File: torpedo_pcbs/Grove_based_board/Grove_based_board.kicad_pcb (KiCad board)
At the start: 2 copper layers, 85 x 27.5 mm, 11 parts, among them IC1 ICM-20948, J1 503480-2200, J2 503480-2200, J3 503480-0440, J4 503480-0440, J5 S8B-EH

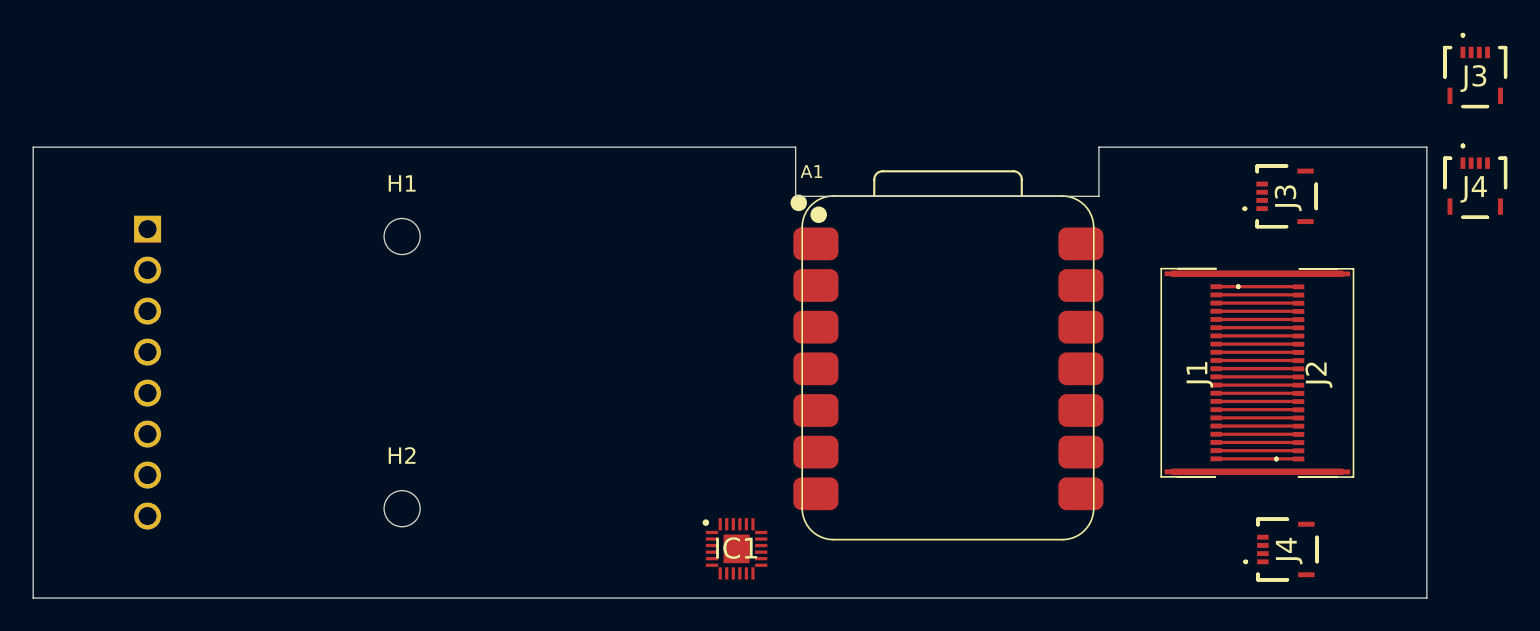
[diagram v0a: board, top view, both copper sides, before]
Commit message: save feb21
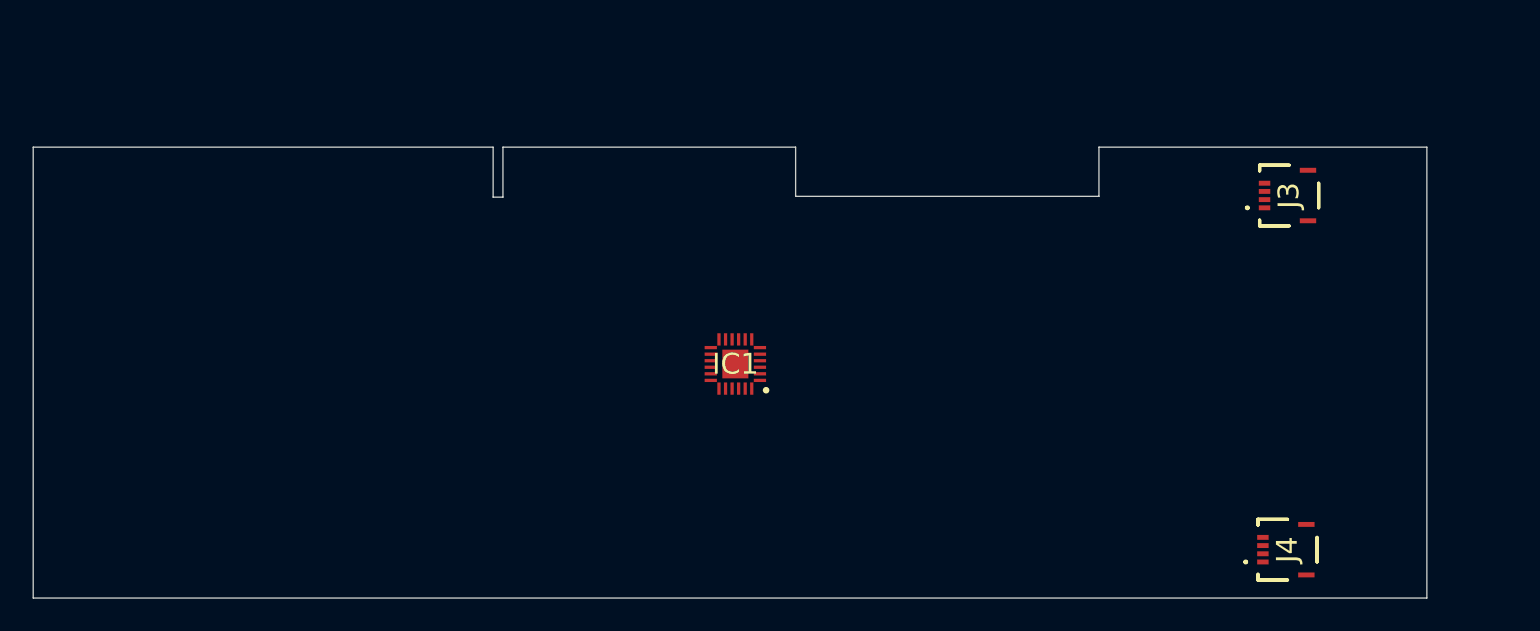
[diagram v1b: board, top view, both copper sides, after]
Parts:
- removed A1: XIAO ESP32S3, board_board_connection:XIAO ESP32S3 SMD
- removed H1, H2: MountingHole, MountingHole:MountingHole_2.2mm_M2
- removed J1, J2: 503480-2200, SamacSys_Parts:5034802200
- removed the J3 at (176.4, 85.0)
- removed the J3 at (187.9, 77.7)
- removed the J4 at (187.9, 84.5)
- removed the J4 at (176.5, 106.5)
- removed J5: S8B-EH, SamacSys_Parts:SHDRRA8W64P0X250_1X8_2250X820X420P
- added J3: 503480-0440, SamacSys_Parts:5034800440, F.Cu at (176.6, 85.0)
- added J4: 503480-0440, SamacSys_Parts:5034800440, F.Cu at (176.5, 106.5)
- moved IC1 11.3 mm to (142.8, 95.2), turned to 180 degrees
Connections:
- IC1 pad 10: unconnected-(IC1-REGOUT-Pad10) -> Net-(IC1-REGOUT)
- IC1 pad 11: unconnected-(IC1-FSYNC-Pad11) -> GND
- IC1 pad 12: unconnected-(IC1-INT1-Pad12) -> IMU_INT
- IC1 pad 13: unconnected-(IC1-VDD-Pad13) -> +3.3V
- IC1 pad 18: unconnected-(IC1-GND-Pad18) -> GND
- IC1 pad 20: unconnected-(IC1-RESV_2-Pad20) -> GND
- IC1 pad 22: unconnected-(IC1-NCS-Pad22) -> +3.3V
- IC1 pad 23: unconnected-(IC1-SCL_/_SCLK-Pad23) -> SCL2
- IC1 pad 24: unconnected-(IC1-SDA_/_SDI-Pad24) -> SDA2
- IC1 pad 8: unconnected-(IC1-VDDIO-Pad8) -> +1V8
- IC1 pad 9: unconnected-(IC1-SDO_/_AD0-Pad9) -> GND
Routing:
- net GND: track 20.7 -> 0.00 mm
- net Net-(J1-Pad1): track 5.03 -> 0.00 mm
- net Net-(J1-Pad9): track 5.02 -> 0.00 mm
- net Net-(J1-Pad8): track 5.02 -> 0.00 mm
- net Net-(J1-Pad7): track 5.02 -> 0.00 mm
- net Net-(J1-Pad6): track 5.02 -> 0.00 mm
- net Net-(J1-Pad5): track 5.02 -> 0.00 mm
- net Net-(J1-Pad4): track 5.02 -> 0.00 mm
- net Net-(J1-Pad3): track 5.02 -> 0.00 mm
- net Net-(J1-Pad22): track 5.02 -> 0.00 mm
- net Net-(J1-Pad21): track 5.02 -> 0.00 mm
- net Net-(J1-Pad20): track 5.02 -> 0.00 mm
- net Net-(J1-Pad2): track 5.02 -> 0.00 mm
- net Net-(J1-Pad19): track 5.02 -> 0.00 mm
- net Net-(J1-Pad18): track 5.02 -> 0.00 mm
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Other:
- outline, holes or cut-outs redrawn
- copper layers 2 -> 4

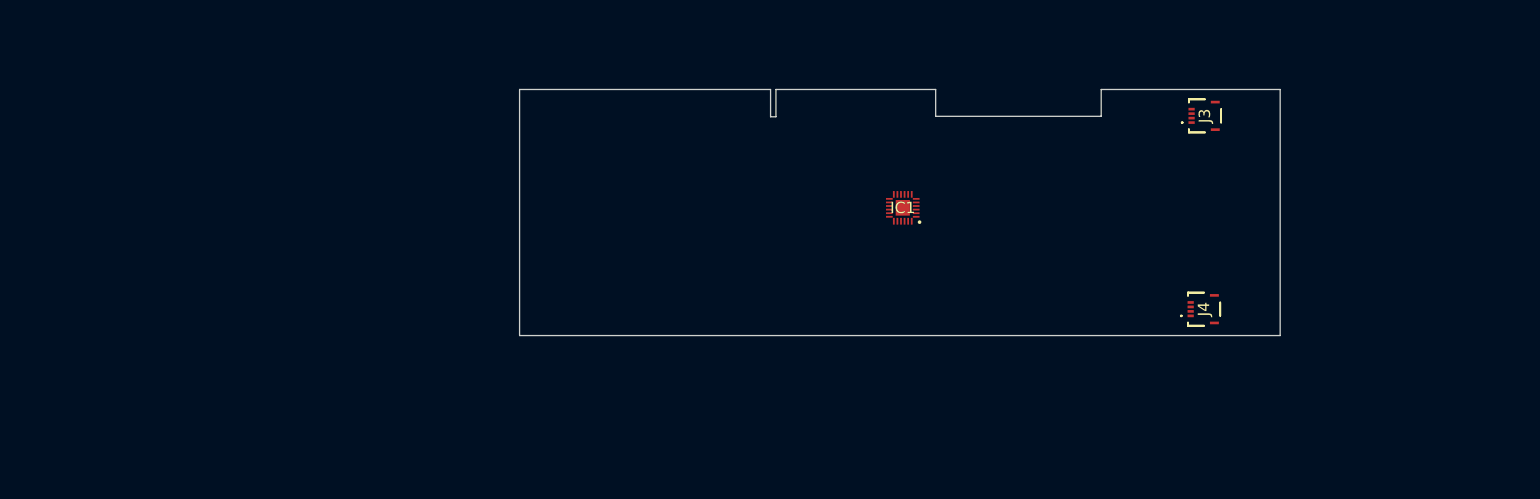
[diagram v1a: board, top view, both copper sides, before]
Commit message: feb23 updates
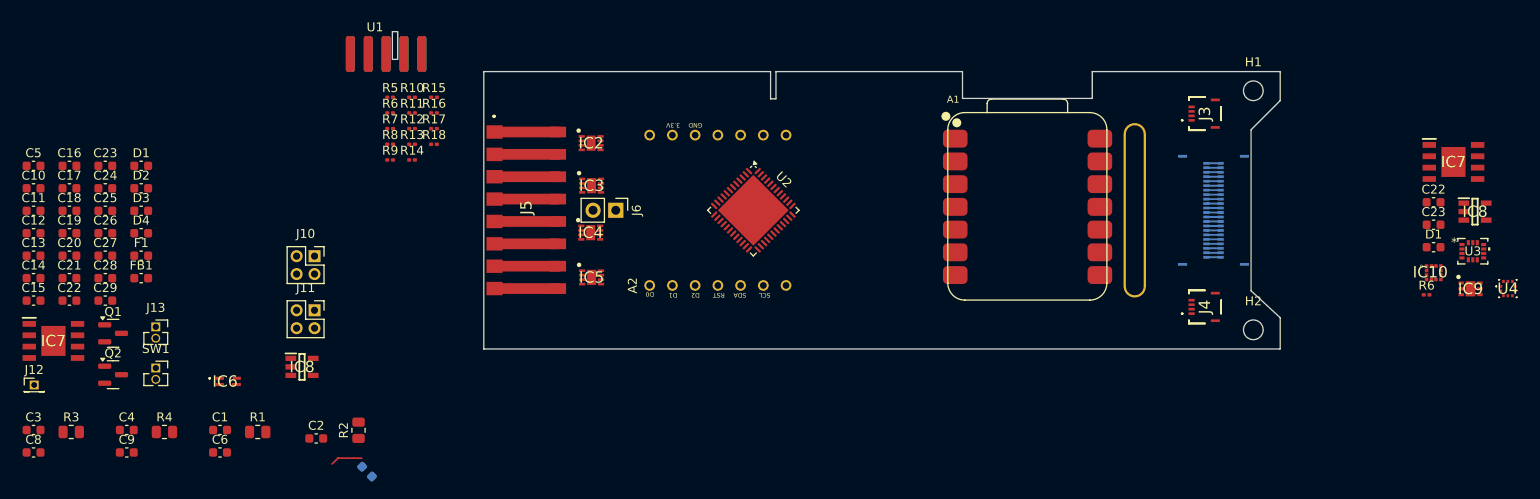
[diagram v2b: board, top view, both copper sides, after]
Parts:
- removed IC1: ICM-20948, SamacSys_Parts:QFN40P300X300X105-25N-D
- added A1: XIAO ESP32S3, board_board_connection:XIAO ESP32S3 SMD, F.Cu at (156.8, 95.1)
- added A2: Grove AI Vision Module V2, board_board_connection:Grove conn, F.Cu at (114.5, 95.5)
- added C1: 0.1μF, Capacitor_SMD:C_0603_1608Metric, F.Cu at (66.5, 120.1)
- added C10: 1μF, Capacitor_SMD:C_0603_1608Metric, F.Cu at (45.7, 93.0)
- added C11: 2.2μF, Capacitor_SMD:C_0603_1608Metric, F.Cu at (45.7, 95.6)
- added C12: 0.1μF, Capacitor_SMD:C_0603_1608Metric, F.Cu at (45.7, 98.1)
- added C13: 10μF, Capacitor_SMD:C_0603_1608Metric, F.Cu at (45.7, 100.6)
- added C14: 0.1μF, Capacitor_SMD:C_0603_1608Metric, F.Cu at (45.7, 103.1)
- added C15: 0.1μF, Capacitor_SMD:C_0603_1608Metric, F.Cu at (45.7, 105.6)
- added C16: 0.1μF, Capacitor_SMD:C_0603_1608Metric, F.Cu at (49.7, 90.5)
- added C17: 0.1μF, Capacitor_SMD:C_0603_1608Metric, F.Cu at (49.7, 93.0)
- added C18: 1μF, Capacitor_SMD:C_0603_1608Metric, F.Cu at (49.7, 95.6)
- added C19: 10nF, Capacitor_SMD:C_0603_1608Metric, F.Cu at (49.7, 98.1)
- added C2: 0.1μF, Capacitor_SMD:C_0603_1608Metric, F.Cu at (77.3, 121.0)
- added C20: 1μF, Capacitor_SMD:C_0603_1608Metric, F.Cu at (49.7, 100.6)
- added C21: 0.1μF, Capacitor_SMD:C_0603_1608Metric, F.Cu at (49.7, 103.1)
- added C22: 10μF, Capacitor_SMD:C_0603_1608Metric, F.Cu at (202.1, 94.6)
- added C22: 10μF, Capacitor_SMD:C_0603_1608Metric, F.Cu at (49.7, 105.6)
- added C23: 10μF, Capacitor_SMD:C_0603_1608Metric, F.Cu at (202.1, 97.1)
- added C23: 10μF, Capacitor_SMD:C_0603_1608Metric, F.Cu at (53.7, 90.5)
- added C24: ??μF, Capacitor_SMD:C_0603_1608Metric, F.Cu at (53.7, 93.0)
- added C25: 1μF, Capacitor_SMD:C_0603_1608Metric, F.Cu at (53.7, 95.6)
- added C26: ??μF, Capacitor_SMD:C_0603_1608Metric, F.Cu at (53.7, 98.1)
- added C27: 0.1μF, Capacitor_SMD:C_0603_1608Metric, F.Cu at (53.7, 100.6)
- added C28: 22nF, Capacitor_SMD:C_0603_1608Metric, F.Cu at (53.7, 103.1)
- added C29: 22nF, Capacitor_SMD:C_0603_1608Metric, F.Cu at (53.7, 105.6)
- added C3: 0.1μF, Capacitor_SMD:C_0603_1608Metric, F.Cu at (45.7, 120.1)
- added C4: 0.1μF, Capacitor_SMD:C_0603_1608Metric, F.Cu at (56.1, 120.1)
- added C5: 0.1μF, Capacitor_SMD:C_0603_1608Metric, F.Cu at (45.7, 90.5)
- added C6: 47μF, Capacitor_SMD:C_0603_1608Metric, F.Cu at (66.5, 122.6)
- added C7: 47μF, Capacitor_SMD:C_0603_1608Metric, B.Cu at (83.0, 124.7)
- added C8: 47μF, Capacitor_SMD:C_0603_1608Metric, F.Cu at (45.7, 122.6)
- added C9: 47μF, Capacitor_SMD:C_0603_1608Metric, F.Cu at (56.1, 122.6)
- added D1: LED, Capacitor_SMD:C_0603_1608Metric, F.Cu at (57.7, 90.5)
- added D1: LED, Capacitor_SMD:C_0603_1608Metric, F.Cu at (202.1, 99.6)
- added D2: LED, Capacitor_SMD:C_0603_1608Metric, F.Cu at (57.7, 93.0)
- added D3: LED, Capacitor_SMD:C_0603_1608Metric, F.Cu at (57.7, 95.6)
- added D4: LED, Capacitor_SMD:C_0603_1608Metric, F.Cu at (57.7, 98.1)
- added F1: Fuse, Capacitor_SMD:C_0603_1608Metric, F.Cu at (57.7, 100.6)
- added FB1: FerriteBead, Capacitor_SMD:C_0603_1608Metric, F.Cu at (57.7, 103.1)
- added H1: MountingHole, MountingHole:MountingHole_2.2mm_M2, F.Cu at (182.0, 82.1)
- added H2: MountingHole, MountingHole:MountingHole_2.2mm_M2, F.Cu at (182.0, 108.9)
- added H3: 22pin->15pin Adapter Slot, MountingEquipment:slot, F.Cu at (168.8, 95.5)
- added IC10: LIS2MDLTR: Magnetometer, SamacSys_Parts:LGA-12, F.Cu at (202.2, 102.5)
- added IC2: DRV8213DSGR, SamacSys_Parts:SON50P200X200X80-9N, F.Cu at (108.0, 88.0)
- added IC3: DRV8213DSGR, SamacSys_Parts:SON50P200X200X80-9N, F.Cu at (108.0, 92.8)
- added IC4: DRV8213DSGR, SamacSys_Parts:SON50P200X200X80-9N, F.Cu at (108.0, 98.0)
- added IC5: DRV8213DSGR, SamacSys_Parts:SON50P200X200X80-9N, F.Cu at (108.0, 103.0)
- added IC6: VEML6040A3OG, SamacSys_Parts:VEML6040A3OG, F.Cu at (68.4, 114.6)
- added IC7: AP7362-33SP-13, SamacSys_Parts:SOIC127P600X150-9N, F.Cu at (47.9, 110.1)
- added IC7: AP7362-33SP-13: Batt->3.3V, SamacSys_Parts:SOIC127P600X150-9N, F.Cu at (204.4, 90.1)
- added IC8: TPS76918DBVR, SamacSys_Parts:SOT95P280X145-5N, F.Cu at (75.7, 113.0)
- added IC8: TPS76918DBVR: 3.3V->1.8V, SamacSys_Parts:SOT95P280X145-5N, F.Cu at (206.8, 95.7)
- added IC9: TPS60150DRVR: 3.3V->5V, SamacSys_Parts:SON65P200X200X80-7N, F.Cu at (206.3, 104.3)
- added J1: 503480-2200, SamacSys_Parts:5034802200, B.Cu at (178.1, 95.5)
- added J10: UART Comms, Connector_PinSocket_2.00mm:PinSocket_2x02_P2.00mm_Vertical, F.Cu at (77.1, 100.6)
- added J11: LCD Screen, Connector_PinSocket_2.00mm:PinSocket_2x02_P2.00mm_Vertical, F.Cu at (77.1, 106.7)
- added J12: Conn_01x01, Connector_PinHeader_1.27mm:PinHeader_1x01_P1.27mm_Vertical, F.Cu at (45.8, 115.0)
- added J13: Fan, Connector_PinSocket_1.27mm:PinSocket_1x02_P1.27mm_Vertical, F.Cu at (59.3, 108.5)
- added J2: 503480-2200, SamacSys_Parts:5034802200, B.Cu at (177.0, 95.5)
- added J5: Push-in Terminals, SamacSys_Parts:009276008021106, F.Cu at (100.8, 95.5)
- added J6: LiHV (3.8V), Connector_PinHeader_2.54mm:PinHeader_1x02_P2.54mm_Vertical, F.Cu at (110.8, 95.5)
- added Q1: BSS138, Package_TO_SOT_SMD:SOT-23, F.Cu at (54.6, 109.2)
- added Q2: BSS138, Package_TO_SOT_SMD:SOT-23, F.Cu at (54.6, 113.9)
- added R1: 8.45k, Resistor_SMD:R_0805_2012Metric, F.Cu at (70.7, 120.3)
- added R10: R, Resistor_SMD:R_0201_0603Metric, F.Cu at (88.0, 82.9)
- added R11: R, Resistor_SMD:R_0201_0603Metric, F.Cu at (88.0, 84.6)
- added R12: 10k, Resistor_SMD:R_0201_0603Metric, F.Cu at (88.0, 86.4)
- added R13: 20k, Resistor_SMD:R_0201_0603Metric, F.Cu at (88.0, 88.1)
- added R14: 10k, Resistor_SMD:R_0201_0603Metric, F.Cu at (88.0, 89.9)
- added R15: 10k, Resistor_SMD:R_0201_0603Metric, F.Cu at (90.4, 82.9)
- added R16: 10k, Resistor_SMD:R_0201_0603Metric, F.Cu at (90.4, 84.6)
- added R17: 10k, Resistor_SMD:R_0201_0603Metric, F.Cu at (90.4, 86.4)
- added R18: ???, Resistor_SMD:R_0201_0603Metric, F.Cu at (90.4, 88.1)
- added R2: 8.45k, Resistor_SMD:R_0805_2012Metric, F.Cu at (82.0, 120.1)
- added R3: 8.45k, Resistor_SMD:R_0805_2012Metric, F.Cu at (49.9, 120.3)
- added R4: 8.45k, Resistor_SMD:R_0805_2012Metric, F.Cu at (60.3, 120.3)
- added R5: 10k, Resistor_SMD:R_0201_0603Metric, F.Cu at (85.5, 82.9)
- added R6: R, Resistor_SMD:R_0201_0603Metric, F.Cu at (201.4, 105.0)
- added R6: R, Resistor_SMD:R_0201_0603Metric, F.Cu at (85.5, 84.6)
- added R7: 2.2k, Resistor_SMD:R_0201_0603Metric, F.Cu at (85.5, 86.4)
- added R8: 2.2k, Resistor_SMD:R_0201_0603Metric, F.Cu at (85.5, 88.1)
- added R9: R, Resistor_SMD:R_0201_0603Metric, F.Cu at (85.5, 89.9)
- added SW1: SW_SPDT, Connector_PinSocket_1.27mm:PinSocket_1x02_P1.27mm_Vertical, F.Cu at (59.3, 113.1)
- added U1: STLINK-V3MINIE Edge Connector, edge connector:STLINK-V3MINIE conn, F.Cu at (85.1, 78.0)
- added U2: STM32G473CBU6, Package_DFN_QFN:QFN-48-1EP_7x7mm_P0.5mm_EP5.6x5.6mm, F.Cu at (126.1, 95.5)
- added U3: LSM6DSOTR: Acc+Gyro+Temp, SamacSys_Parts:LGA-14L_2P5X3X0P86_STM, F.Cu at (206.5, 100.1)
- added U4: ILPS22QS: Air Pressure+Temp, SamacSys_Parts:LPS22HHTR, F.Cu at (210.4, 104.2)
- moved J4 0.27 mm to (176.6, 106.3)
- moved J3 0.25 mm to (176.6, 84.7)
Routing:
- net /Motor driver0/OUT1: track 0.00 -> 7.70 mm
- net /Motor driver3/OUT2: track 0.00 -> 7.10 mm
- net /Motor driver3/OUT1: track 0.00 -> 7.10 mm
- net /Motor driver2/OUT2: track 0.00 -> 7.10 mm
- net /Motor driver1/OUT1: track 0.00 -> 7.10 mm
- net /Motor driver0/OUT2: track 0.00 -> 7.10 mm
- net /Motor driver2/OUT1: track 0.00 -> 7.10 mm
- net /Motor driver1/OUT2: track 0.00 -> 7.10 mm
- net MOTOR1_IPROPI: track 0.00 -> 3.56 mm
- net Net-(J1-Pad14): track 0.00 -> 1.60 mm
- net Net-(J1-Pad20): track 0.00 -> 1.60 mm
- net Net-(J1-Pad7): track 0.00 -> 1.60 mm
- net Net-(J1-Pad19): track 0.00 -> 1.60 mm
- net Net-(J1-Pad16): track 0.00 -> 1.60 mm
- net Net-(J1-Pad10): track 0.00 -> 1.60 mm
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- added copper zone on In2.Cu, net +3.3V
- added copper zone on In2.Cu, net +BATT
- added copper zone on In1.Cu, net GND
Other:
- board size 85 x 27.5 mm -> 89 x 31 mm
